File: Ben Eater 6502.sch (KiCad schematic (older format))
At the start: 10 parts, among them SW1 Reset, U1 W65C02SxP, U2 4011, U3 28C256, U4 4011, U5 W65C22SxP

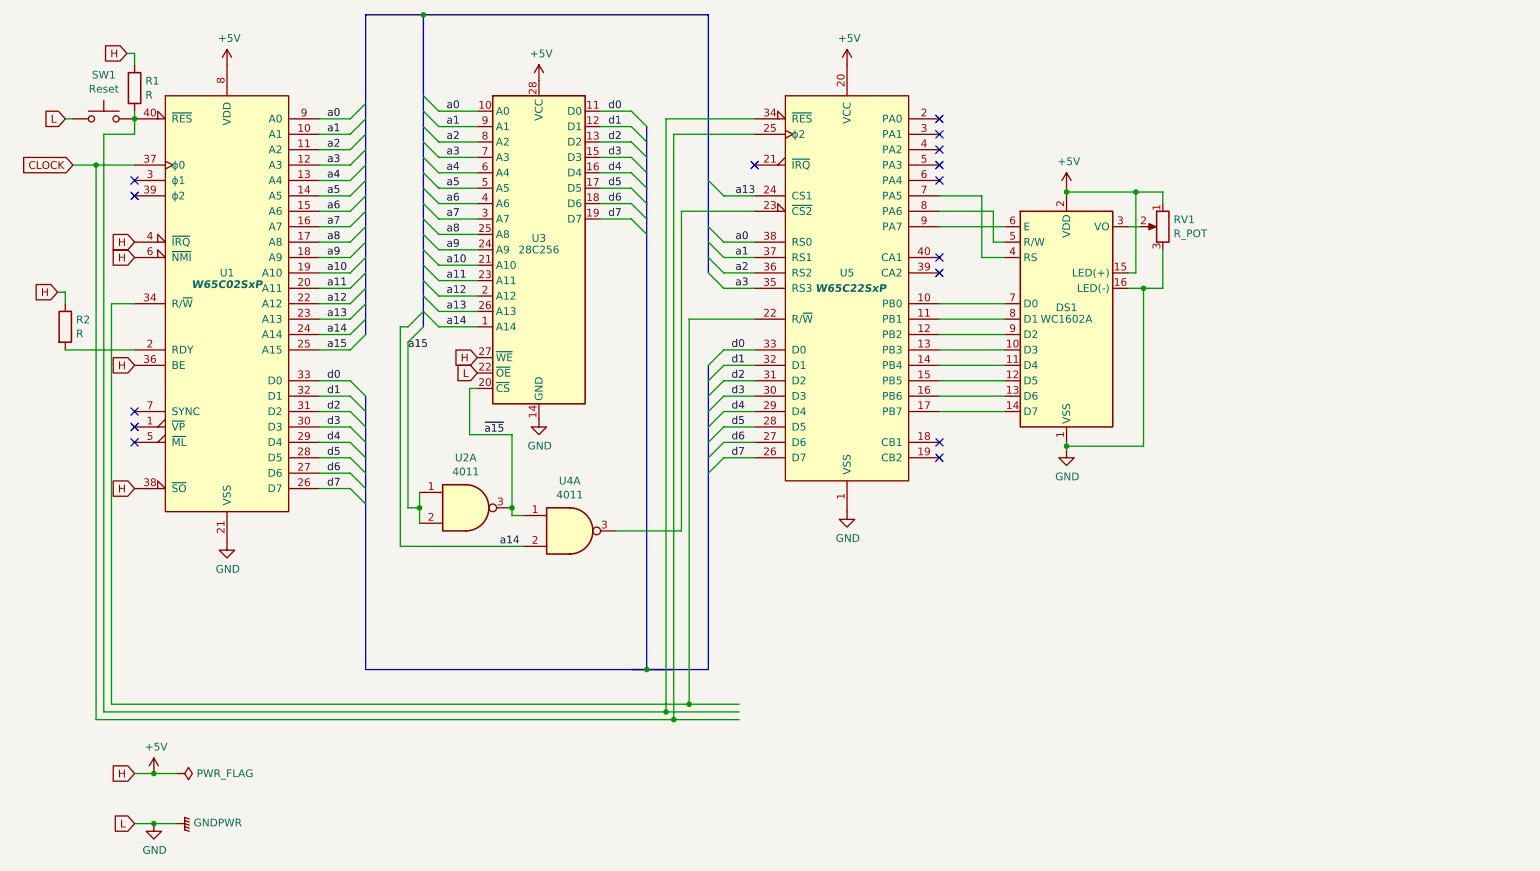
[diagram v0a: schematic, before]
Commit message: Stage 4
Add RAM
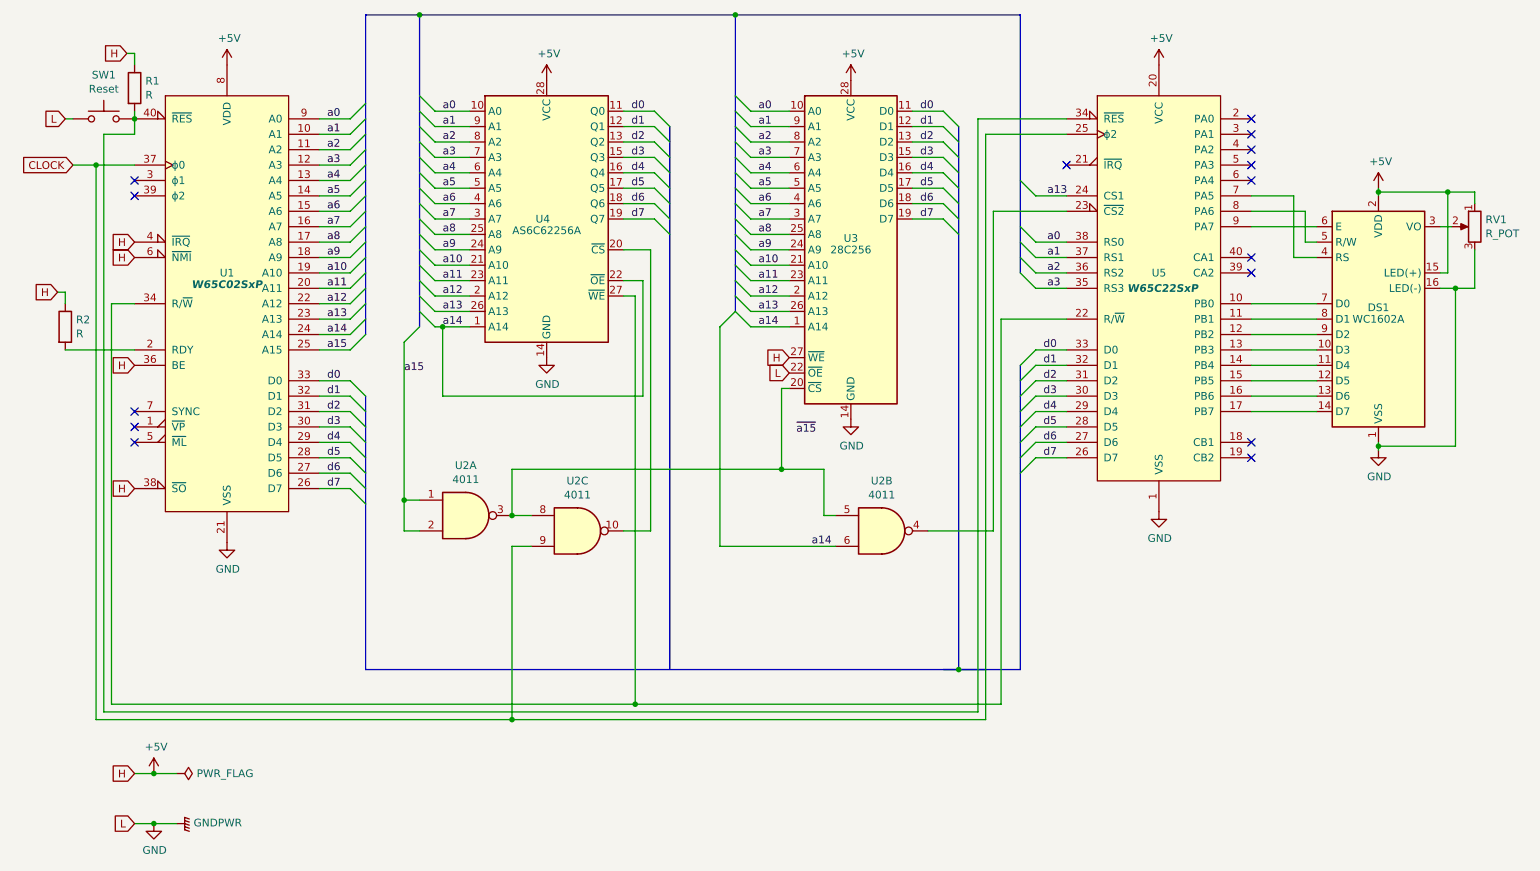
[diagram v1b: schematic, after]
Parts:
- added unit 3 of U2
- added U4: AS6C62256A, Package_DIP:DIP-28_W15.24mm, symbol Memory_RAM:KM62256CLP
- renumbered U4 to U2
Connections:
- net +5V: now also U4.28 (VCC)
- net CLOCK: now also U2.9
- net GND: now also U4.14 (GND)
- net a0: now also U4.10 (A0)
- net a1: now also U4.9 (A1)
- net a10: now also U4.21 (A10)
- net a11: now also U4.23 (A11)
- net a12: now also U4.2 (A12)
- net a13: now also U4.26 (A13)
- net a14: now also U2.6, U4.1 (A14), U4.22 (~OE); no longer U2.2
- net a2: now also U4.8 (A2)
- net a3: now also U4.7 (A3)
- net a4: now also U4.6 (A4)
- net a5: now also U4.5 (A5)
- net a6: now also U4.4 (A6)
- net a7: now also U4.3 (A7)
- net a8: now also U4.25 (A8)
- net a9: now also U4.24 (A9)
- net d0: now also U4.11 (Q0)
- net d1: now also U4.12 (Q1)
- net d2: now also U4.13 (Q2)
- net d3: now also U4.15 (Q3)
- net d4: now also U4.16 (Q4)
- net d5: now also U4.17 (Q5)
- net d6: now also U4.18 (Q6)
- net d7: now also U4.19 (Q7)
- net ~a15: no longer U2.1, U2.3, U3.20 (~CS)
- net at U1.34 (R/~W), U5.22 (R/~W): now also U4.27 (~WE)
- net at U5.23 (~CS2): now also U2.4; no longer U2.3
- new net: U2.3, U2.5, U2.8, U3.20 (~CS)
- new net: U2.10, U4.20 (~CS)
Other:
- moved on the sheet: DS1, RV1, U2A, U3, U5
